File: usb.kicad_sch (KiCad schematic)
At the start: 10 parts, among them J7 USB_C_Receptacle_USB2.0, U28 USBLC6-4SC6

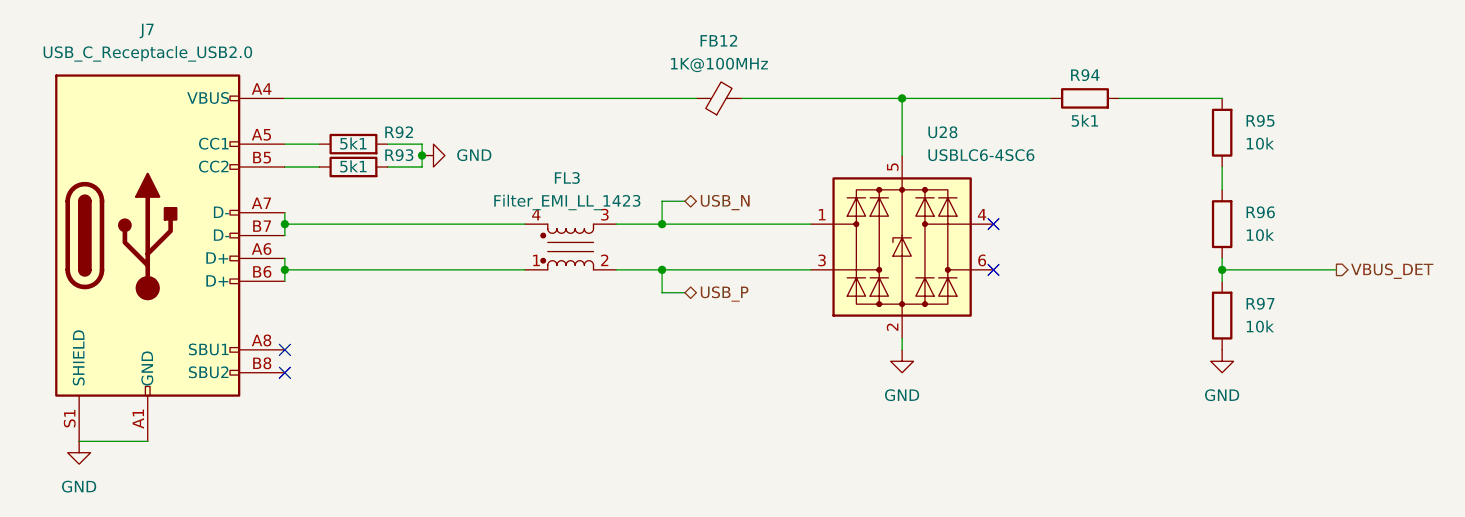
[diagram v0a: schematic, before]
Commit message: v 0.2 schematics
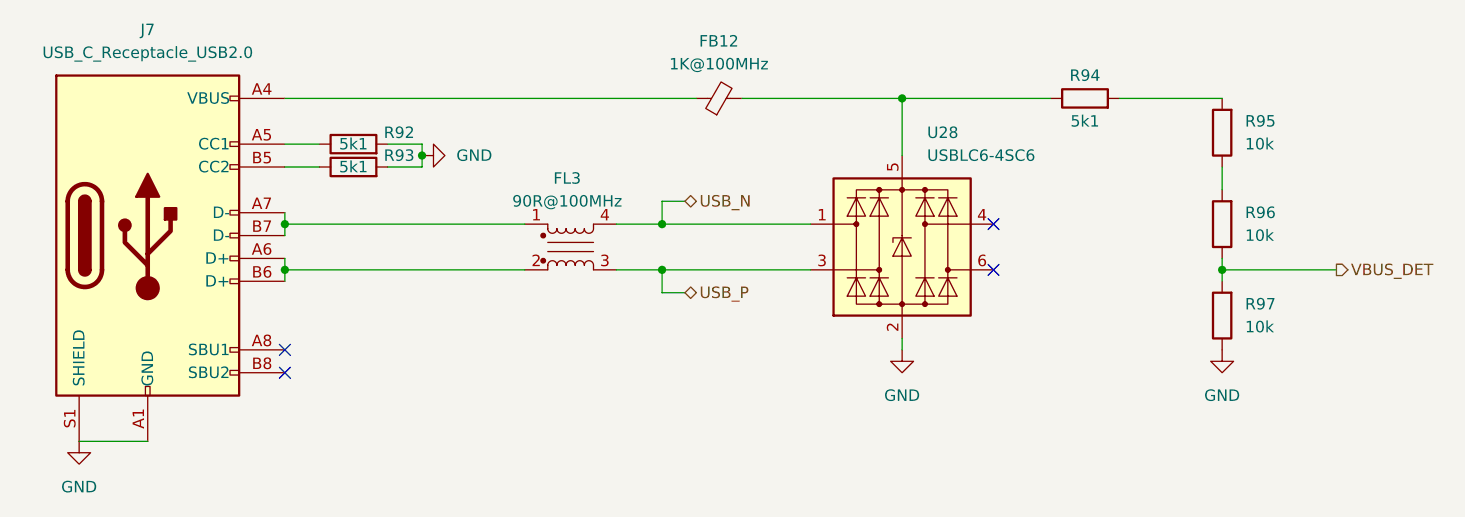
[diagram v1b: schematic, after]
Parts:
- removed FL3: Filter_EMI_LL_1423, Inductor_SMD:L_CommonModeChoke_Coilcraft_0603USB, symbol kirdy:Filter_EMI_LL_1423
- added FL3: 90R@100MHz, Inductor_SMD:L_CommonModeChoke_Coilcraft_0603USB, symbol Device:Filter_EMI_LL_1423
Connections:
- net USB_N: now also FL3.4
- net USB_P: now also FL3.3
- net at J7.A6 (D+), J7.B6 (D+): now also FL3.2
- net at J7.A7 (D-), J7.B7 (D-): now also FL3.1
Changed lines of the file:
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@@
     (pin "1")
-  )
-  (symbol (lib_id "kirdy:Filter_EMI_LL_1423") (at 175.26 104.14 0) (mirror x) (unit 1)
-    (in_bom yes) (on_board yes) (fields_autoplaced)
-    (property "Reference" "FL3" (id 0) (at 174.879 96.52 0))
-    (property "Value" "Filter_EMI_LL_1423" (id 1) (at 174.879 99.06 0))
-    (property "Footprint" "Inductor_SMD:L_CommonModeChoke_Coilcraft_0603USB" (id 2) (at 175.26 105.156 0)
-      (effects (font (size 1.27 1.27)) hide)
-    )
-    (property "Datasheet" "~" (id 3) (at 175.26 105.156 0)
-      (effects (font (size 1.27 1.27)) hide)
-    )
-    (property "MFR_PN" "ACM-0603-121-T" (id 4) (at 175.26 104.14 0)
-      (effects (font (size 1.27 1.27)) hide)
-    )
-    (pin "1")
-    (pin "2")
-    (pin "3")
-    (pin "4")
   )
   (symbol (lib_id "Connector:USB_C_Receptacle_USB2.0") (at 128.27 102.87 0) (unit 1)
@@
     (pin "2")
   )
+  (symbol (lib_id "Device:Filter_EMI_LL_1423") (at 175.26 104.14 0) (mirror x) (unit 1)
+    (in_bom yes) (on_board yes) (fields_autoplaced)
+    (property "Reference" "FL3" (id 0) (at 174.879 96.52 0))
+    (property "Value" "90R@100MHz" (id 1) (at 174.879 99.06 0))
+    (property "Footprint" "Inductor_SMD:L_CommonModeChoke_Coilcraft_0603USB" (id 2) (at 175.26 97.79 0)
+      (effects (font (size 1.27 1.27)) hide)
+    )
+    (property "Datasheet" "~" (id 3) (at 175.26 105.156 90)
+      (effects (font (size 1.27 1.27)) hide)
+    )
+    (property "MFR_PN" "0603USB-222MLC" (id 4) (at 175.26 104.14 0)
+      (effects (font (size 1.27 1.27)) hide)
+    )
+    (property "MFR_PN_ALT" "0603USB-951MLC" (id 5) (at 175.26 104.14 0)
+      (effects (font (size 1.27 1.27)) hide)
+    )
+    (pin "1")
+    (pin "2")
+    (pin "3")
+    (pin "4")
+  )
   (symbol (lib_id "Device:R") (at 151.13 95.25 90) (unit 1)

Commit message: complete placement
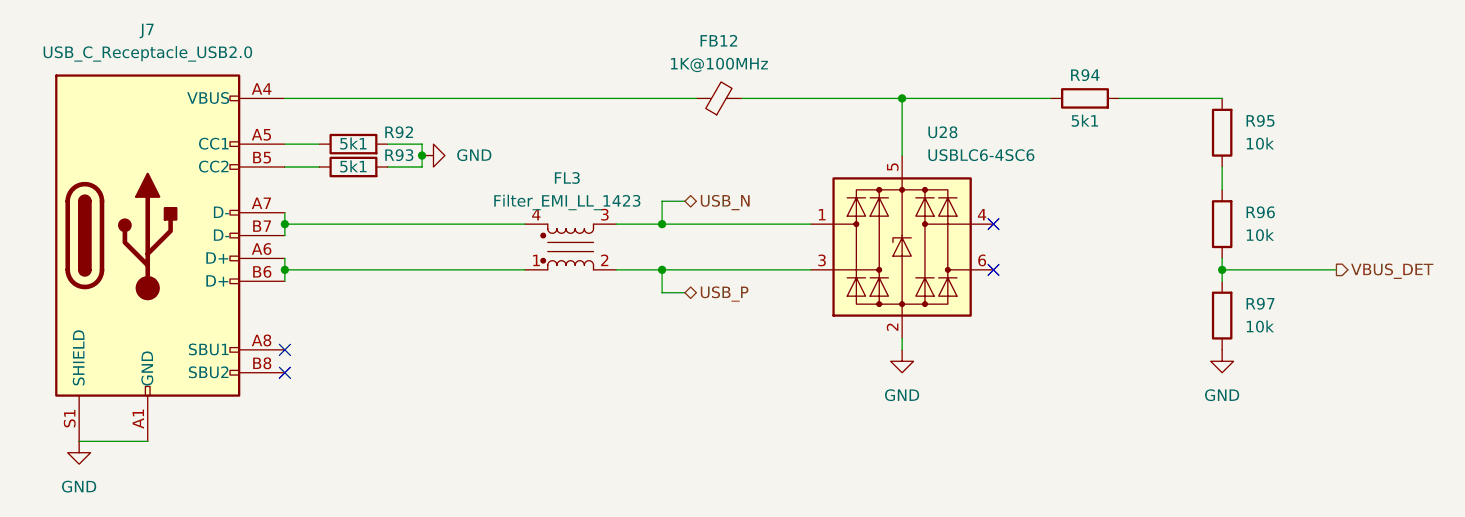
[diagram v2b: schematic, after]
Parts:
- removed FL3: 90R@100MHz, Inductor_SMD:L_CommonModeChoke_Coilcraft_0603USB, symbol Device:Filter_EMI_LL_1423
- added FL3: Filter_EMI_LL_1423, Inductor_SMD:L_CommonModeChoke_Coilcraft_0603USB, symbol kirdy:Filter_EMI_LL_1423
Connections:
- net USB_N: now also FL3.3
- net USB_P: now also FL3.2
- net at J7.A6 (D+), J7.B6 (D+): now also FL3.1
- net at J7.A7 (D-), J7.B7 (D-): now also FL3.4
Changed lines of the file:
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@@
     (pin "1")
+  )
+  (symbol (lib_id "kirdy:Filter_EMI_LL_1423") (at 175.26 104.14 0) (mirror x) (unit 1)
+    (in_bom yes) (on_board yes) (fields_autoplaced)
+    (property "Reference" "FL3" (id 0) (at 174.879 96.52 0))
+    (property "Value" "Filter_EMI_LL_1423" (id 1) (at 174.879 99.06 0))
+    (property "Footprint" "Inductor_SMD:L_CommonModeChoke_Coilcraft_0603USB" (id 2) (at 175.26 105.156 0)
+      (effects (font (size 1.27 1.27)) hide)
+    )
+    (property "Datasheet" "~" (id 3) (at 175.26 105.156 0)
+      (effects (font (size 1.27 1.27)) hide)
+    )
+    (property "MFR_PN" "ACM-0603-121-T" (id 4) (at 175.26 104.14 0)
+      (effects (font (size 1.27 1.27)) hide)
+    )
+    (pin "1")
+    (pin "2")
+    (pin "3")
+    (pin "4")
   )
   (symbol (lib_id "Connector:USB_C_Receptacle_USB2.0") (at 128.27 102.87 0) (unit 1)
@@
     (pin "2")
   )
-  (symbol (lib_id "Device:Filter_EMI_LL_1423") (at 175.26 104.14 0) (mirror x) (unit 1)
-    (in_bom yes) (on_board yes) (fields_autoplaced)
-    (property "Reference" "FL3" (id 0) (at 174.879 96.52 0))
-    (property "Value" "90R@100MHz" (id 1) (at 174.879 99.06 0))
-    (property "Footprint" "Inductor_SMD:L_CommonModeChoke_Coilcraft_0603USB" (id 2) (at 175.26 97.79 0)
-      (effects (font (size 1.27 1.27)) hide)
-    )
-    (property "Datasheet" "~" (id 3) (at 175.26 105.156 90)
-      (effects (font (size 1.27 1.27)) hide)
-    )
-    (property "MFR_PN" "0603USB-222MLC" (id 4) (at 175.26 104.14 0)
-      (effects (font (size 1.27 1.27)) hide)
-    )
-    (property "MFR_PN_ALT" "0603USB-951MLC" (id 5) (at 175.26 104.14 0)
-      (effects (font (size 1.27 1.27)) hide)
-    )
-    (pin "1")
-    (pin "2")
-    (pin "3")
-    (pin "4")
-  )
   (symbol (lib_id "Device:R") (at 151.13 95.25 90) (unit 1)
